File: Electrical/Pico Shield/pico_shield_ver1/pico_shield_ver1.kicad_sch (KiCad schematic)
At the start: 39 parts, among them U2 ULN2003A, U3 ULN2003A

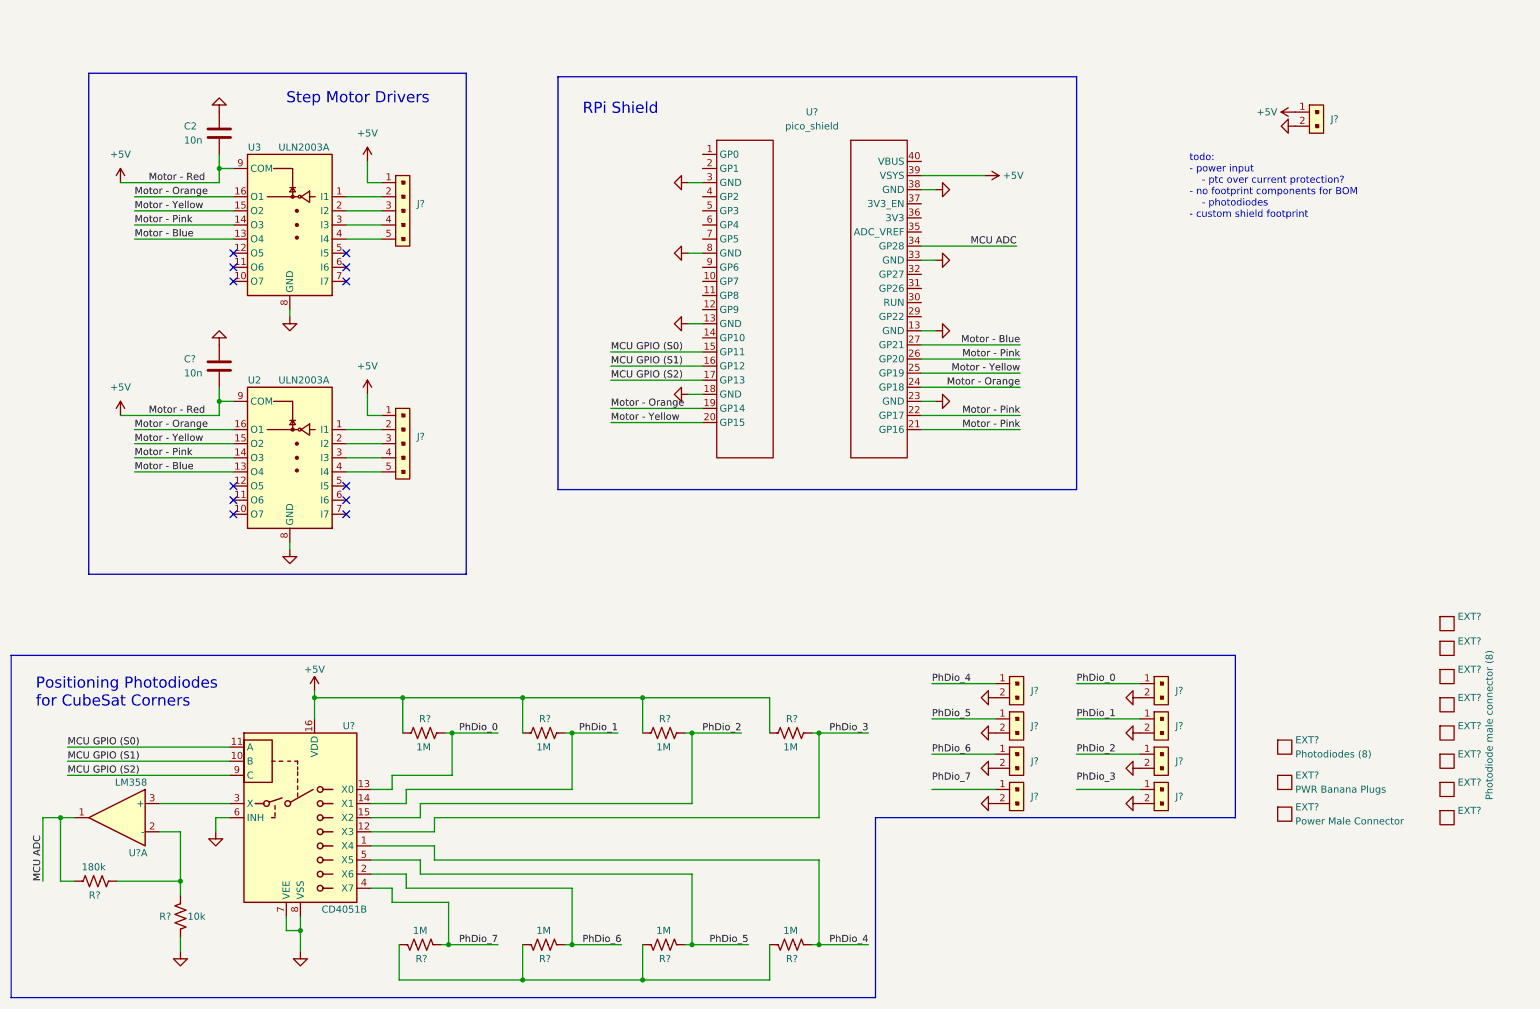
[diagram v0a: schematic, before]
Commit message: progress
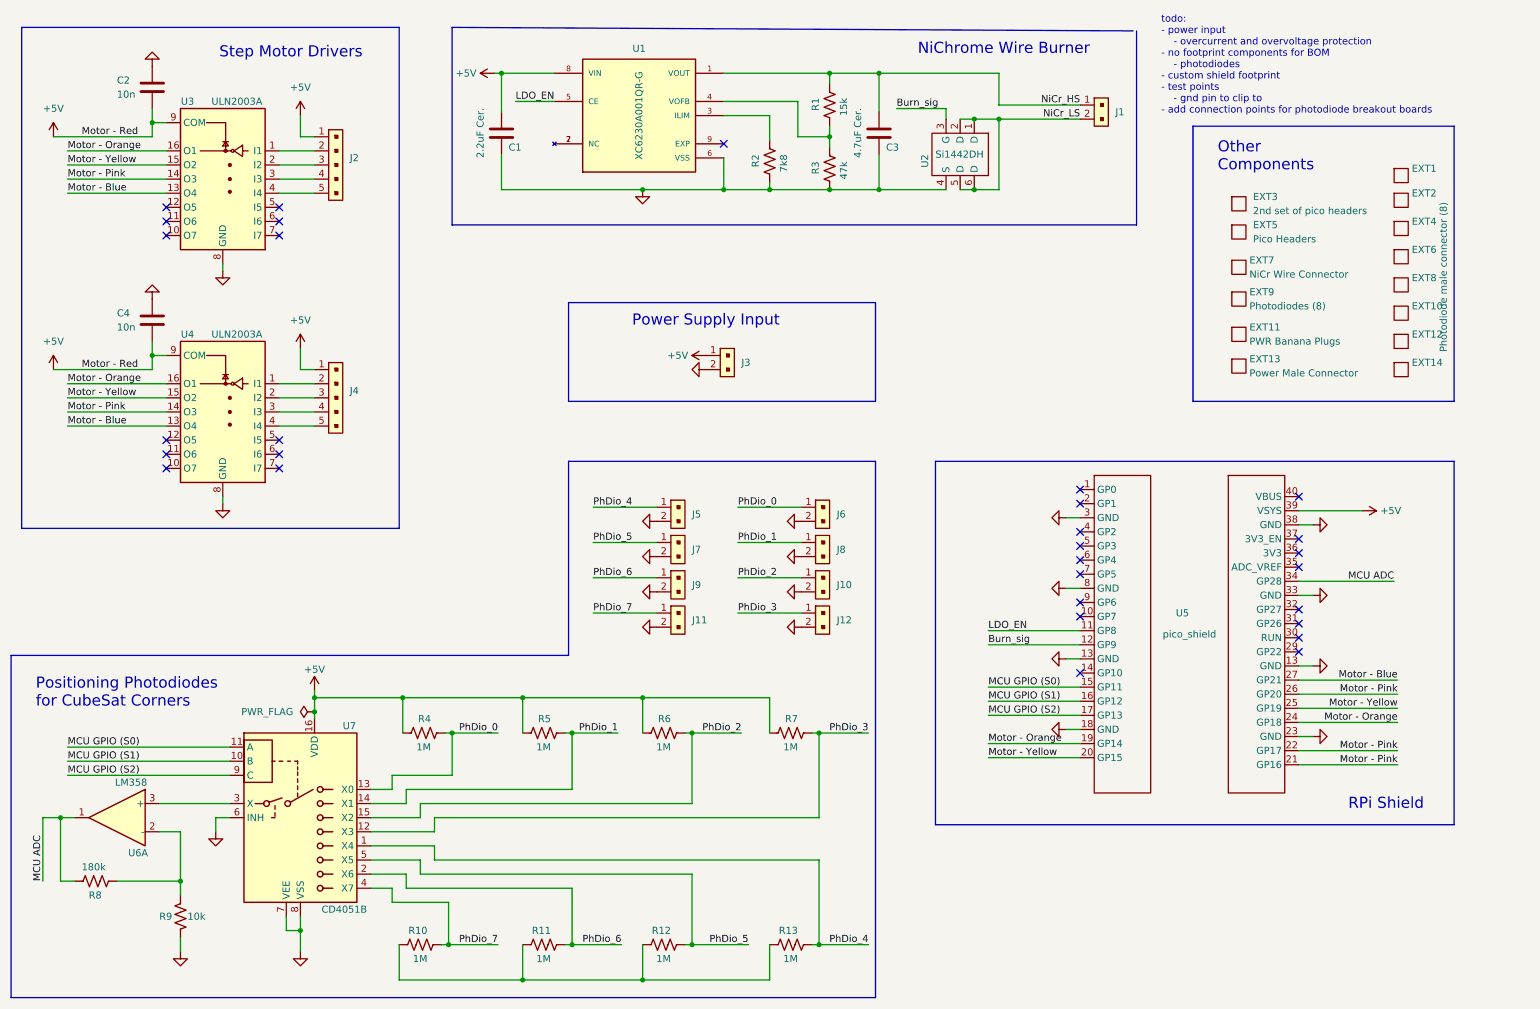
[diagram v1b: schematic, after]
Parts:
- removed C?: 10n, symbol Device:C
- removed R? (x7): 1M, symbol Device:R_US
- removed U2: ULN2003A, symbol Transistor_Array:ULN2003A
- added C1: 2.2uF Cer., Capacitor_SMD:C_0805_2012Metric, symbol Device:C
- added C3: 4.7uF Cer., Capacitor_SMD:C_0805_2012Metric, symbol Device:C
- added C4: 10n, Capacitor_SMD:C_0805_2012Metric, symbol Device:C
- added EXT3: 2nd set of pico headers, 0_custom:EXT_no_footprint, symbol 0_custom:{lt}name{gt}
- added EXT5: Pico Headers, 0_custom:EXT_no_footprint, symbol 0_custom:{lt}name{gt}
- added EXT7: NiCr Wire Connector, 0_custom:EXT_no_footprint, symbol 0_custom:{lt}name{gt}
- added J1: 644752-2, Miles Added:644752-2_TYC, symbol dk_Rectangular-Connectors-Headers-Male-Pins:B2B-PH-K-S_LF__SN_
- added R1: 15k, Resistor_SMD:R_0805_2012Metric_Pad1.20x1.40mm_HandSolder, symbol Device:R_US
- added R10, R11, R12, R13, R5, R6, R7: 1M, Resistor_SMD:R_0805_2012Metric_Pad1.20x1.40mm_HandSolder, symbol Device:R_US
- added R2: 7k8, Resistor_SMD:R_0805_2012Metric_Pad1.20x1.40mm_HandSolder, symbol Device:R_US
- added R3: 47k, Resistor_SMD:R_0805_2012Metric_Pad1.20x1.40mm_HandSolder, symbol Device:R_US
- added U1: XC6230A001QR-G, Miles Added:SOIC127P600X175-9N, symbol XC6230A001QR-G:XC6230A001QR-G
- added U2: Si1442DH, Package_TO_SOT_SMD:SOT-363_SC-70-6, symbol 0_custom:Si1442DH
- added U4: ULN2003A, Miles Added:ULN2003ADR2G_OSI, symbol Transistor_Array:ULN2003A
- C2: footprint (none) -> Capacitor_SMD:C_0805_2012Metric; MPN (none) -> 0805YC103MAT2A
- R4: renamed from R?; footprint (none) -> Resistor_SMD:R_0805_2012Metric_Pad1.20x1.40mm_HandSolder; MPN (none) -> RT0805BRD071ML
- R8: renamed from R?; footprint (none) -> Resistor_SMD:R_0805_2012Metric_Pad1.20x1.40mm_HandSolder; MPN (none) -> RC0805FR-07182KL
- R9: renamed from R?; footprint (none) -> Resistor_SMD:R_0805_2012Metric_Pad1.20x1.40mm_HandSolder; MPN (none) -> RMCF0805FT10K0
- U3: footprint (none) -> Miles Added:ULN2003ADR2G_OSI; MPN (none) -> ULN2003ADR2G
- U5: renamed from U?; footprint (none) -> 0_custom:PICO_SHIELD; MPN (none) -> PRT-16279
- U6: renamed from U?; footprint (none) -> Miles Added:M08A-L; MPN (none) -> LM358MX
- U7: renamed from U?; footprint (none) -> Miles Added:PW0016A_L; MPN (none) -> CD4051BQPWRG4Q1
- gave numbers to parts that had none: 22
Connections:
- net +5V: now also C1.1, C4.2, R5.1, R6.1, R7.1, U1.8 (VIN), U4.9 (COM)
- net GND: now also C1.2, C3.2, C4.1, R2.1, R3.1, U1.6 (VSS), U2.4 (S), U4.8 (GND)
- net Motor - Blue: now also U4.13 (O4)
- net Motor - Orange: now also U4.16 (O1)
- net Motor - Pink: now also U4.14 (O3)
- net Motor - Yellow: now also U4.15 (O2)
- net PhDio_1: now also R5.2
- net PhDio_2: now also R6.2
- net PhDio_3: now also J12.1, R7.2
- net PhDio_4: now also R13.2
- net PhDio_5: now also R12.2
- net PhDio_6: now also R11.2
- net PhDio_7: now also J11.1, R10.2
- net at J4.2: now also U4.1 (I1)
- net at J4.3: now also U4.2 (I2)
- net at J4.4: now also U4.3 (I3)
- net at J4.5: now also U4.4 (I4)
- net LDO_EN: now reaches U5.11 (GP8)
- net LDO_EN: now also U1.5 (CE)
- net Burn_sig: now reaches U5.12 (GP9)
- net Burn_sig: now also U2.3 (G)
- new net: R1.1, R3.2, U1.4 (VOFB)
- new net: R10.1, R11.1, R12.1, R13.1
- new net: U1.2 (NC), U1.7 (NC)
- new net: R2.2, U1.3 (ILIM)
- new net NiCr_HS: C3.1, J1.1, R1.2, U1.1 (VOUT)
- new net NiCr_LS: J1.2, U2.1 (D), U2.2 (D), U2.5 (D), U2.6 (D)
- no-connect marks 12 -> 30
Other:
- note added: "NiChrome Wire Burner"
- note added: "Other Components"
- note added: "Power Supply Input"
- note added: "todo: - power input - overcurrent and overvoltage protection - no footprint components for BOM - photodiodes - custom shield footprint - test points - gnd pin to clip to - add connection points for photodiode breakout boards"
- note removed: "todo: - power input - ptc over current protection? - no footprint components for BOM - photodiodes - custom shield footprint"
- company: (none) -> Cal Poly, SLO
- title: (none) -> CubeSat Pi Hat
- moved on the sheet: C2, EXT1, EXT10, EXT11, EXT12, EXT13, EXT14, EXT2, EXT4, EXT6, EXT8, EXT9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
